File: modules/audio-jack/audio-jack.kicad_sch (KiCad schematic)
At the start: 6 parts, among them J1 SJ-43514-SMT-TR

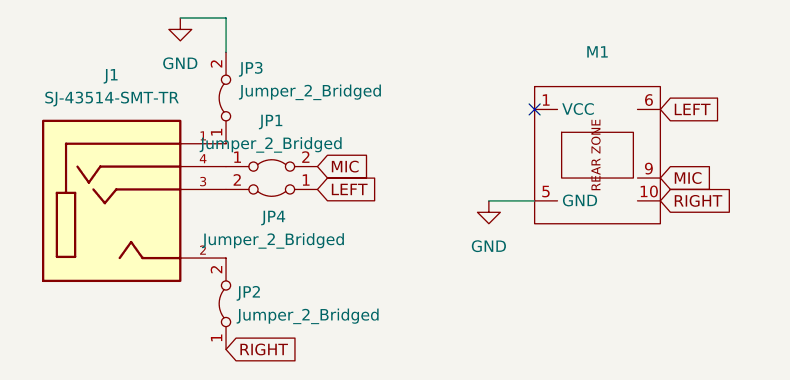
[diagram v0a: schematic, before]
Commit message: Updating all modules
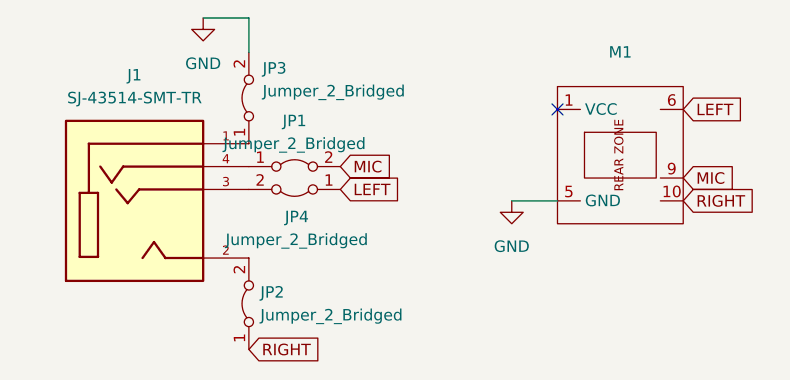
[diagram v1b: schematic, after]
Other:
- moved on the sheet: J1, JP1, JP2, JP3, JP4, M1
